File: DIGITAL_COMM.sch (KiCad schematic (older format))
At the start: 4 parts, among them U5 MCP3004, U6 TC77

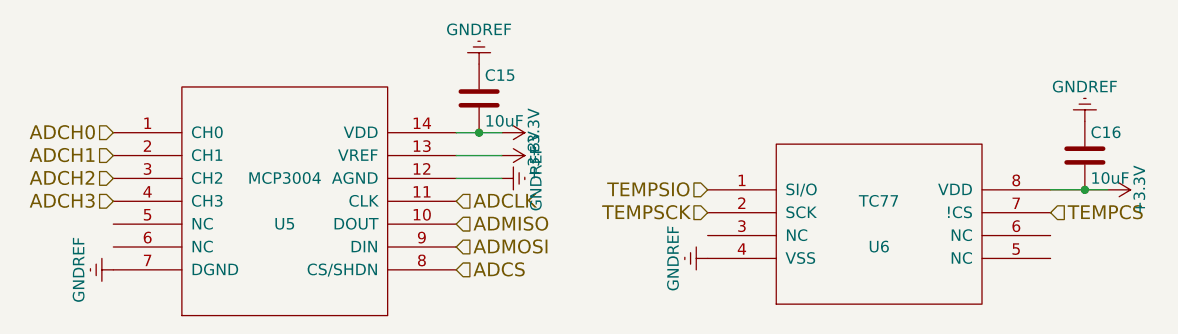
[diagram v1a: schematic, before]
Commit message: small changes
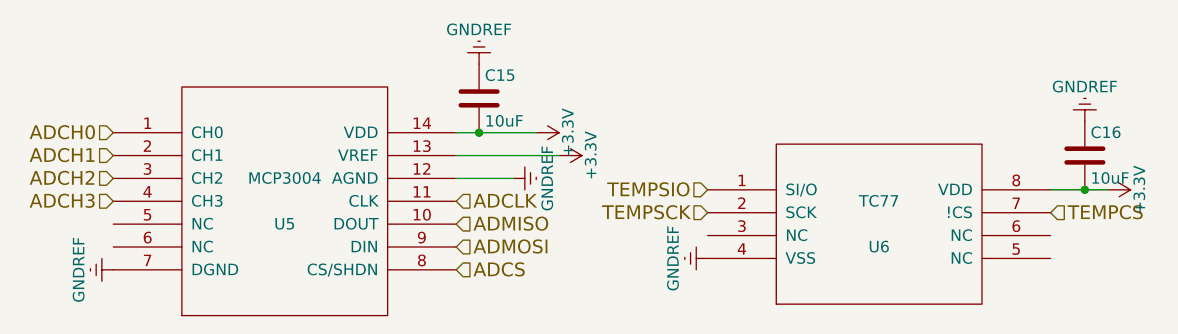
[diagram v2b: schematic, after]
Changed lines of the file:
@@
 LIBS:valves
 LIBS:analog_devices
-LIBS:libs
 LIBS:viztisztito-cache
 EELAYER 25 0
@@
 L +3.3V #PWR036
 U 1 1 561B952F
-P 4500 2300
-F 0 "#PWR036" H 4500 2150 50  0001 C CNN
-F 1 "+3.3V" H 4500 2440 50  0000 C CNN
-F 2 "" H 4500 2300 60  0000 C CNN
-F 3 "" H 4500 2300 60  0000 C CNN
-	1    4500 2300
+P 4650 2300
+F 0 "#PWR036" H 4650 2150 50  0001 C CNN
+F 1 "+3.3V" H 4650 2440 50  0000 C CNN
+F 2 "" H 4650 2300 60  0000 C CNN
+F 3 "" H 4650 2300 60  0000 C CNN
+	1    4650 2300
 	0    1    1    0
 $EndComp
@@
 L GNDREF #PWR039
 U 1 1 561B97FD
-P 4500 2500
-F 0 "#PWR039" H 4500 2250 50  0001 C CNN
-F 1 "GNDREF" H 4500 2350 50  0000 C CNN
-F 2 "" H 4500 2500 60  0000 C CNN
-F 3 "" H 4500 2500 60  0000 C CNN
-	1    4500 2500
+P 4550 2500
+F 0 "#PWR039" H 4550 2250 50  0001 C CNN
+F 1 "GNDREF" H 4550 2350 50  0000 C CNN
+F 2 "" H 4550 2500 60  0000 C CNN
+F 3 "" H 4550 2500 60  0000 C CNN
+	1    4550 2500
 	0    -1   -1   0
 $EndComp
@@
 L +3.3V #PWR040
 U 1 1 561B9824
-P 4500 2400
-F 0 "#PWR040" H 4500 2250 50  0001 C CNN
-F 1 "+3.3V" H 4500 2540 50  0000 C CNN
-F 2 "" H 4500 2400 60  0000 C CNN
-F 3 "" H 4500 2400 60  0000 C CNN
-	1    4500 2400
+P 4750 2400
+F 0 "#PWR040" H 4750 2250 50  0001 C CNN
+F 1 "+3.3V" H 4750 2540 50  0000 C CNN
+F 2 "" H 4750 2400 60  0000 C CNN
+F 3 "" H 4750 2400 60  0000 C CNN
+	1    4750 2400
 	0    1    1    0
 $EndComp
@@
 ADCH1
 Wire Wire Line
-	4300 2300 4500 2300
+	4300 2300 4400 2300
+Wire Wire Line
+	4400 2300 4650 2300
 Connection ~ 4400 2300
 Wire Wire Line
-	4500 2400 4300 2400
+	4750 2400 4300 2400
 Wire Wire Line
-	4300 2500 4500 2500
+	4300 2500 4550 2500
 Wire Wire Line
-	6900 2550 7150 2550
+	6900 2550 7050 2550
+Wire Wire Line
+	7050 2550 7150 2550
 Connection ~ 7050 2550
 Text HLabel 2800 2500 0    60   Input ~ 0
